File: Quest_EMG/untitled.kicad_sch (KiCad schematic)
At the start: 48 parts, among them IC1 OPA2890IDGST, U1 AD8620, U2 INA121UAE4

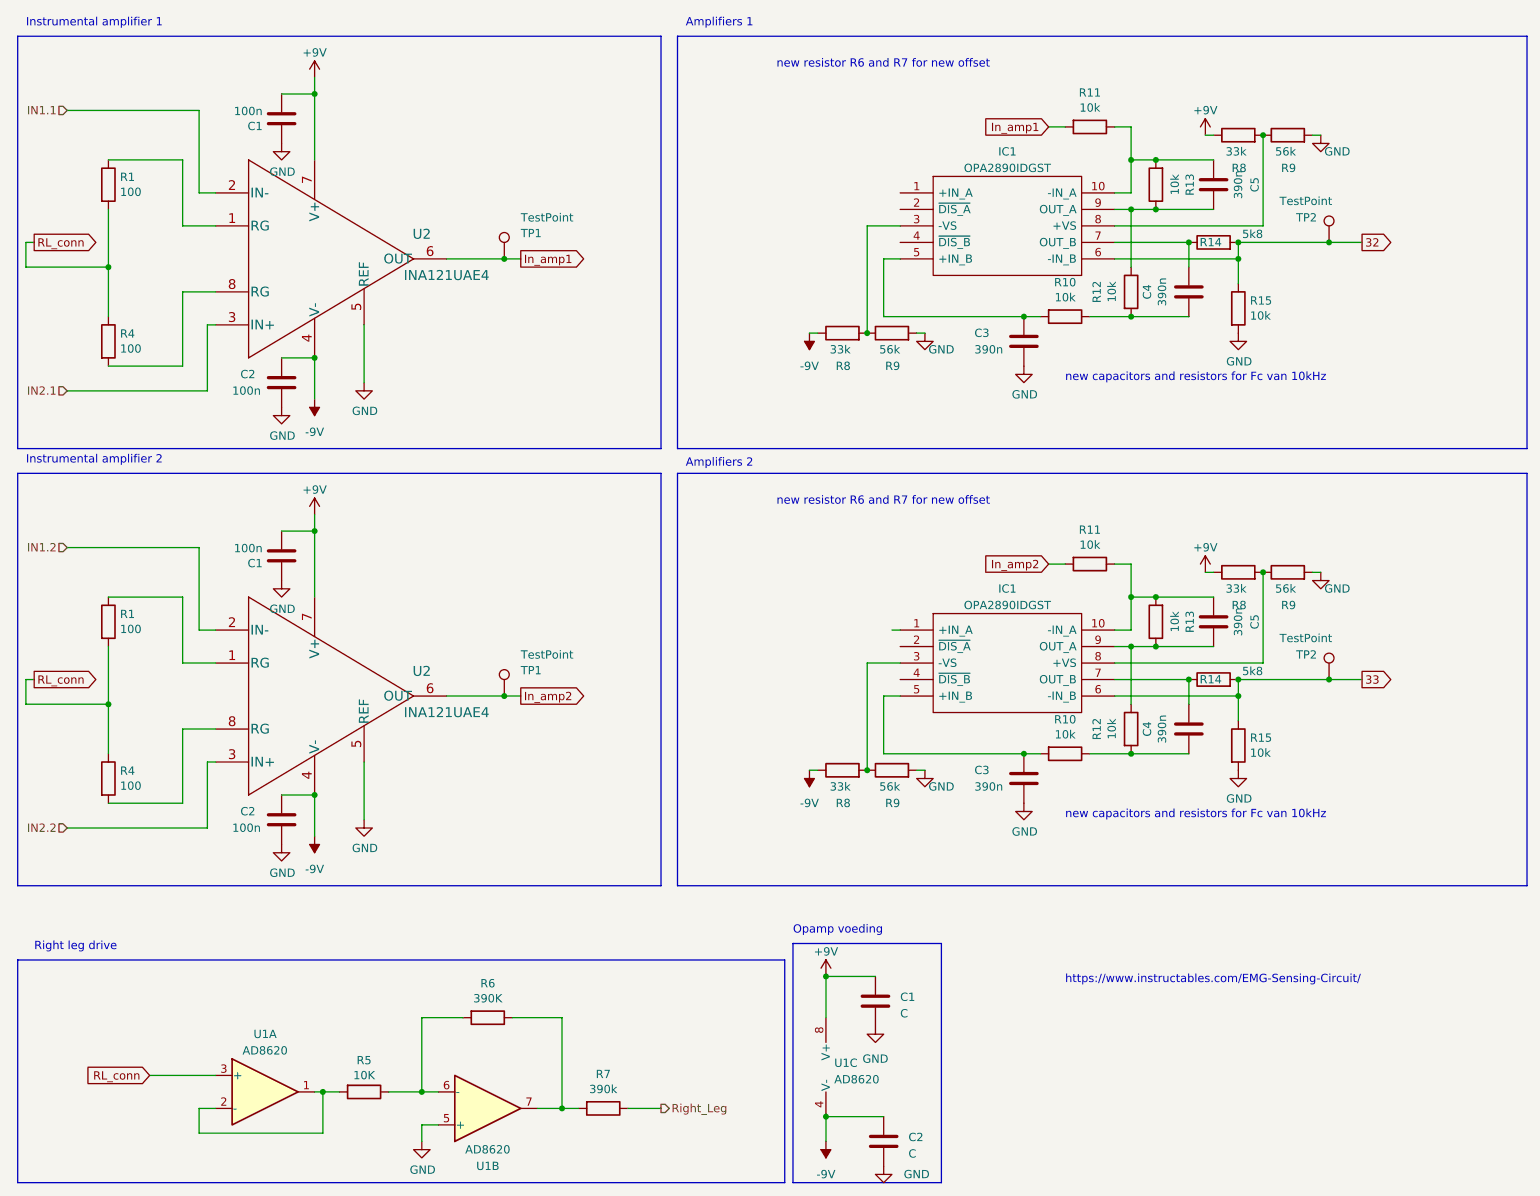
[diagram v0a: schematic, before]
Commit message: forgot something
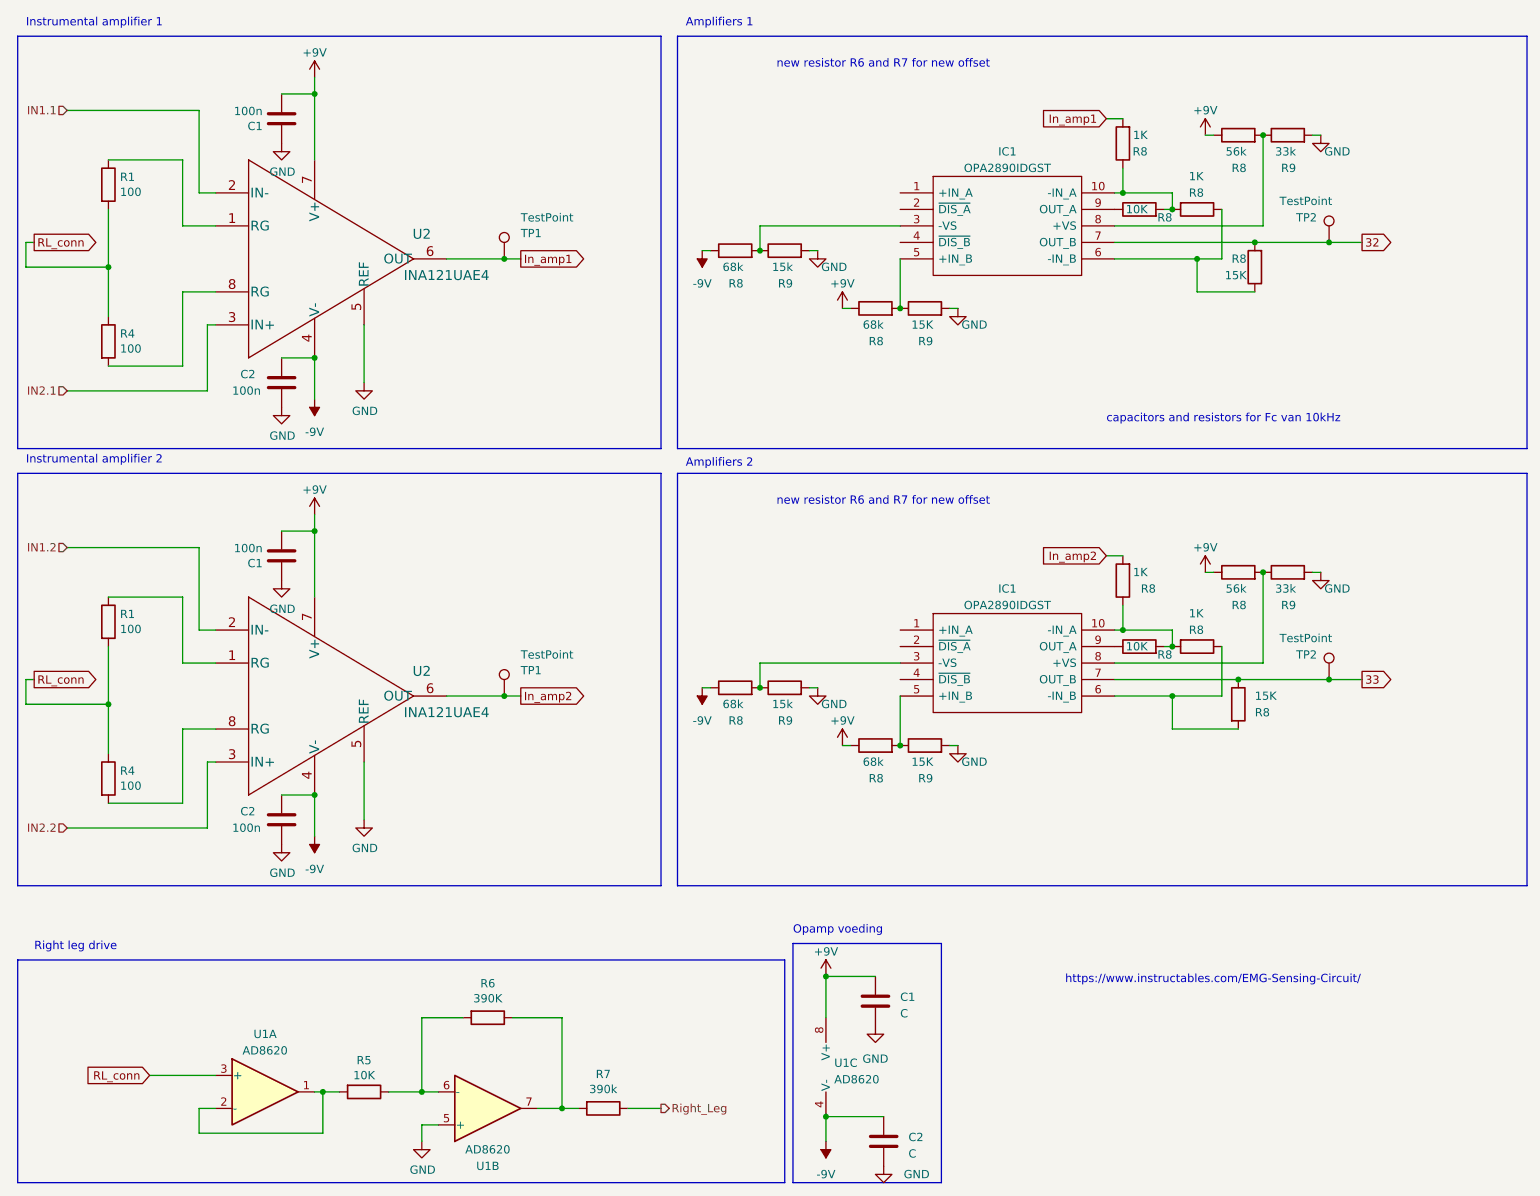
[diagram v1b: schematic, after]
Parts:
- removed C3 (x2), C4 (x2), C5 (x2): 390n, Capacitor_SMD:C_0402_1005Metric, symbol Device:C
- removed R10 (x2), R11 (x2), R12 (x2), R13 (x2), R15 (x2): 10k, Resistor_SMD:R_0402_1005Metric, symbol Device:R
- removed R14 (x2): 5k8, Resistor_SMD:R_0402_1005Metric, symbol Device:R
- removed R8 (x2): 33k, Resistor_SMD:R_0402_1005Metric, symbol Device:R
- removed R9 (x2): 56k, Resistor_SMD:R_0402_1005Metric, symbol Device:R
- added R8 (x4): 1K, Resistor_SMD:R_0402_1005Metric, symbol Device:R
- added R8 (x2), R9 (x2): 15K, Resistor_SMD:R_0402_1005Metric, symbol Device:R
- added R8 (x3): 68k, Resistor_SMD:R_0402_1005Metric, symbol Device:R
- added R8: 56k, Resistor_SMD:R_0402_1005Metric, symbol Device:R
- added R8 (x2): 10K, Resistor_SMD:R_0402_1005Metric, symbol Device:R
- added R9: 15k, Resistor_SMD:R_0402_1005Metric, symbol Device:R
- added R9: 33k, Resistor_SMD:R_0402_1005Metric, symbol Device:R
- R8: value 33k -> 68k
- R8: value 33k -> 56k
- R9: value 56k -> 33k
- R9: value 56k -> 15k
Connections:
- net +9V: now also R8.1, R8.1, R8.1
- net -9V: now also R8.1
- net 32: now also IC1.7 (OUT_B), R8.2; no longer IC1.6 (-IN_B)
- net 33: now also IC1.7 (OUT_B), R8.1; no longer IC1.6 (-IN_B)
- net GND: now also R9.2, R9.2, R9.2, R9.2
- net In_amp1: now also R8.2
- net In_amp2: now also R8.2
- net at IC1.9 (OUT_A): now also R8.1 (x2)
- net at IC1.10 (-IN_A): now also R8.1, R8.2, R8.2 (x2)
- net at IC1.3 (-VS): now also R8.2, R9.1
- net at IC1.5 (+IN_B): now also R8.2, R9.1 (x2)
- net at IC1.8 (+VS): now also R8.2, R9.1
- new net: IC1.6 (-IN_B), R8.1, R8.1
- new net: IC1.6 (-IN_B), R8.1, R8.2
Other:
- note added: "capacitors and resistors for Fc van 10kHz"
- note removed: "new capacitors and resistors for Fc van 10kHz"
- moved on the sheet: R8, R9
